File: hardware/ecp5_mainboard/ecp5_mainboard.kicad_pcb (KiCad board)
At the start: 2 copper layers, 158.1 x 111.2 mm, 498 parts, among them J1 12V_EXT, J10 UART, J11 FLASH, J12 JTAG, J13 Micro_SD_Card, J2 USB_B_Micro, J3 HDMI_A, J4 USB_A, J5 EXT0, J6 EXT1, J7 EXT2, J8 EXT3, J9 PMOD_01, P1 SATA, P2 SATA, P3 PCIe_x4_EDGE, P4 JK0654219NL, Q1 BSH111BKR, Q2 BC850, Q3 BSH111BKR, Q4 BC850, Q5 BSH111BKR, Q6 BSH111BKR, Q7 BSH111BKR, Q8 BSH111BKR, Q9 BSH111BKR, SW1 CHP-081TA, SW2 SW_Push, SW3 SW_Push, SW4 SW_Push, SW5 SW_Push, SW6 SW_Push, U1 MAX811MEUS-T, U10 TPS62823, U12 93AA46B_OT, U13 FT2232H, U14 XUL535150.000JS6I8, U15 ECP5UM5G_85_CABGA756, U16 5P49V6965, U17 TPS2041B, U18 PCA9306, U19 TFP410, U2 LM3880, U20 TPS2041B, U21 KSZ9031RNXCA, U22 USB3300-EZK, U23 AS4C256M16D3, U24 AS4C256M16D3, U25 TPS51200DRC, U26 XL_XO_LVDS, U27 W25Q, U3 TLV75712PDR, U4 TPS565208, U5 LM21212-2, U6 TLV75712PDR, U7 TPS62823, U8 TPS62823, U9 TPS62823, X1 XO32, Y1 25MHz, Y2 25MHz, Y3 24MHz

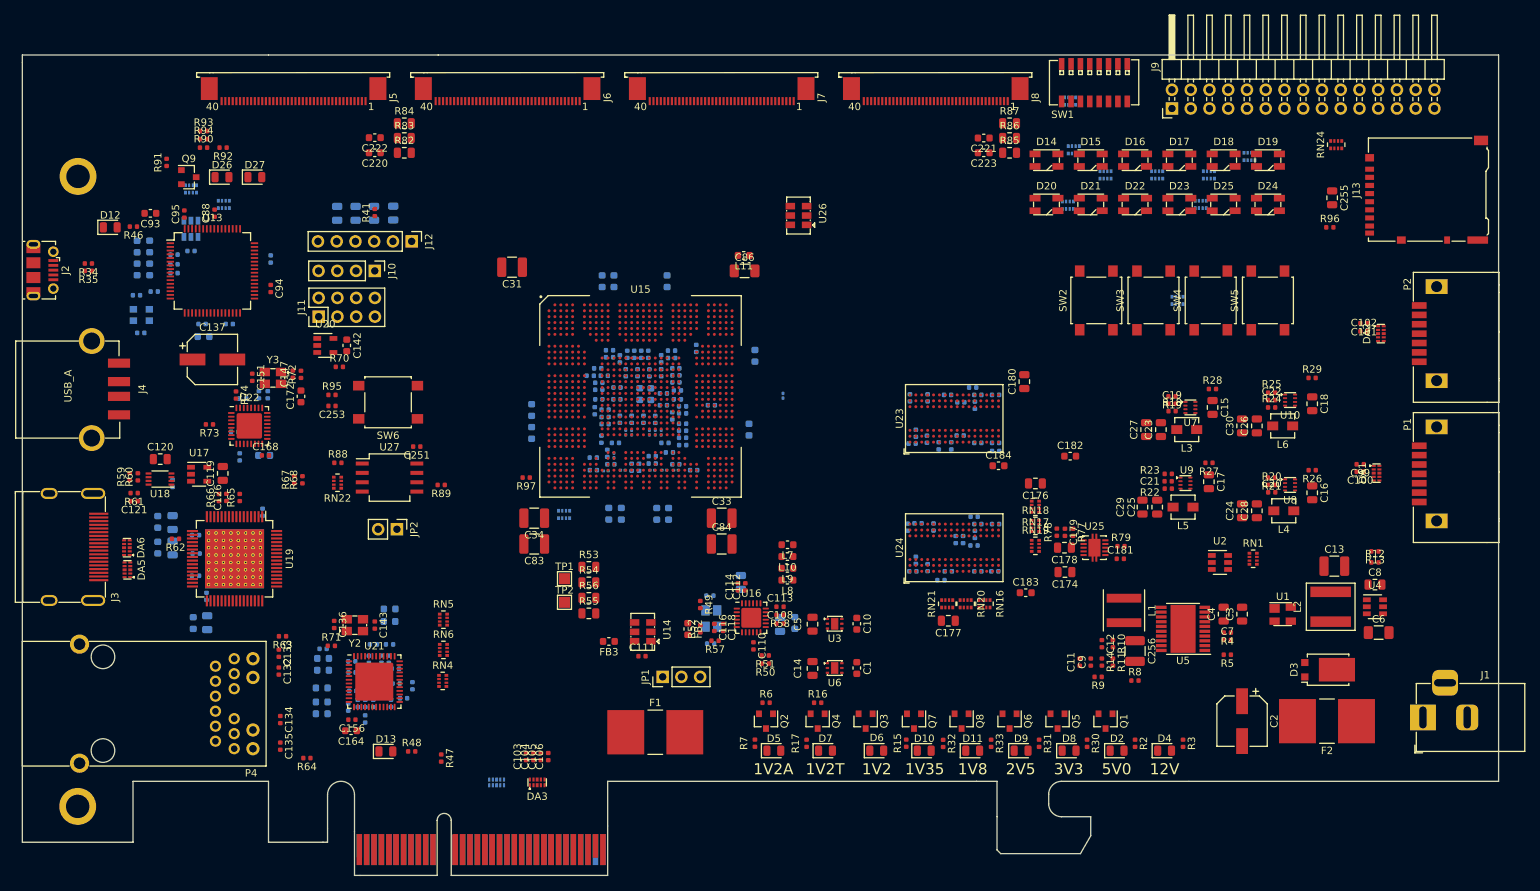
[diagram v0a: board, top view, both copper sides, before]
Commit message: hardware/mainboard: Reduce refdes size to 0.8mm
Signed-off-by: David Shah <dave@ds0.me>
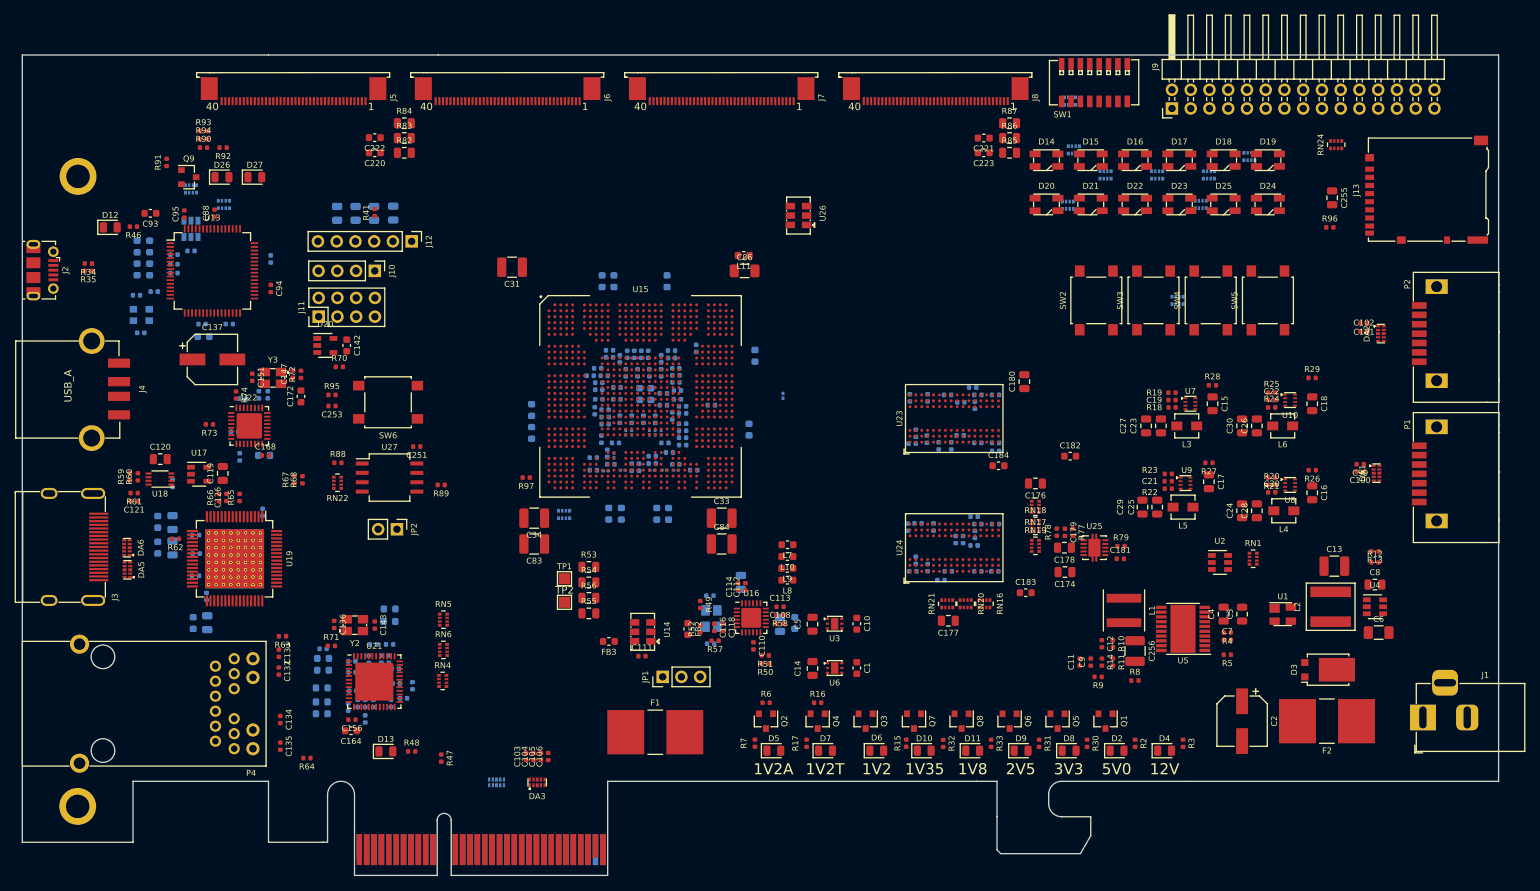
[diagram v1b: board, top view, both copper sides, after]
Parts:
- moved C15 0.50 mm to (201.5, 71.0)
- moved C19 0.50 mm to (196.0, 70.5)
- moved C23 0.50 mm to (194.5, 74.0)
- moved C27 0.50 mm to (192.5, 74.0)
- moved L3 0.50 mm to (198.0, 74.0)
- moved R18 0.50 mm to (196.0, 71.5)
- moved R19 0.50 mm to (196.0, 69.5)
- moved R28 0.50 mm to (201.5, 68.5)
- moved U7 0.50 mm to (198.5, 71.0)
